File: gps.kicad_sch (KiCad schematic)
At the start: 30 parts, among them J5 Micro_SD_Card_Det_Hirose_DM3AT, U10 TPS54560BDDA, U9 74AHCT125

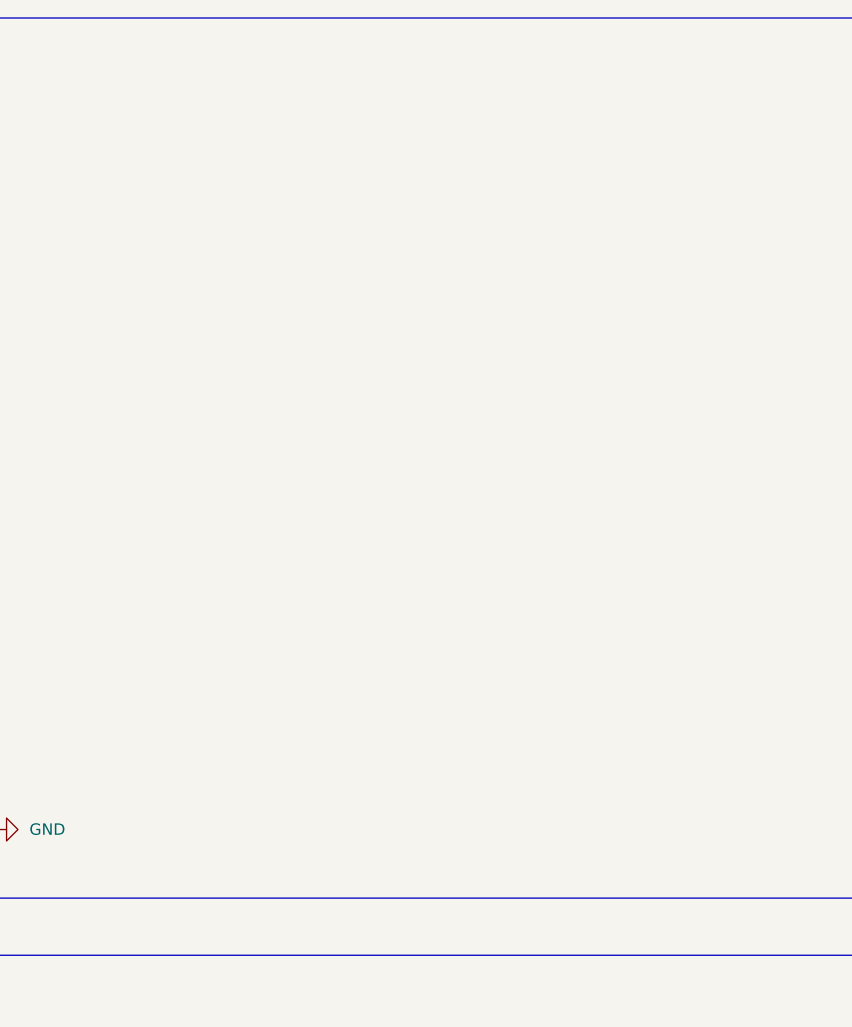
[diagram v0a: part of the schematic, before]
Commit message: Autosave
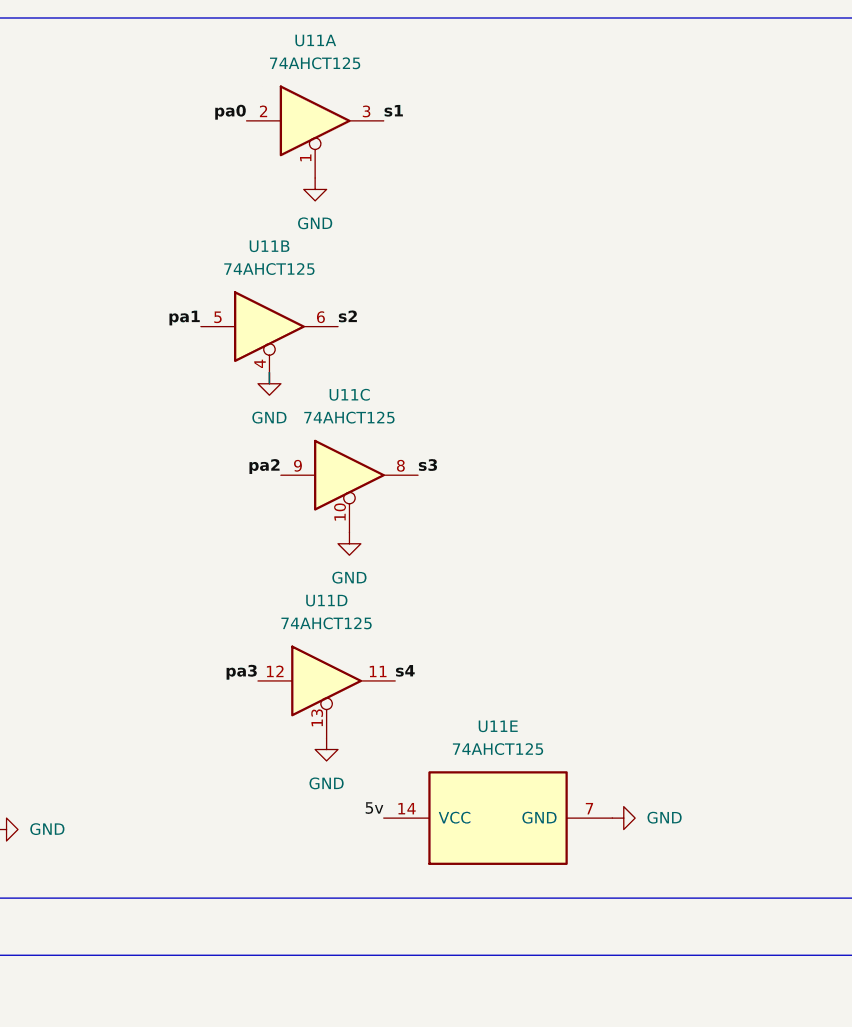
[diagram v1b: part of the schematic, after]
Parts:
- added U11: 74AHCT125, symbol symbols:74AHCT125
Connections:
- net 5v: now also U11.14 (VCC)
- net GND: now also U11.1, U11.10, U11.13, U11.4, U11.7 (GND)
- net pa0: now also U11.2
- net pa1: now also U11.5
- net pa2: now also U11.9
- net pa3: now also U11.12
- net s1: now also U11.3
- net s2: now also U11.6
- net s3: now also U11.8
- net s4: now also U11.11
